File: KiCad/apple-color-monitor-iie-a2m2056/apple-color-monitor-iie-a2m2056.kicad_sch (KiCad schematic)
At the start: 395 parts, among them CN14 Conn_01x04_Pin, CN16 Conn_01x01_Pin, CN20 Conn_01x06_Pin, CN20_plug1 Conn_01x06, CN4 Conn_01x07_Pin, CN4_FRONT1 CN, CN5 Text/Gfx, CN5_FRONT1 Conn_01x02_Socket, CN6 GRN, CN8 Conn_01x02_Pin, CN9 Conn_01x01_Pin, IC102 CD4053B, J101 Jumper_2_Bridged, J102 Jumper_2_Bridged, J103 Jumper_2_Bridged, J104 Jumper_2_Bridged, J106 Jumper_2_Bridged, J107 Jumper_2_Bridged, J108 Jumper_2_Bridged, J109 Jumper_2_Bridged, J110 Jumper_2_Bridged, J111 Jumper_2_Bridged, J112 Jumper_2_Bridged, J113 Jumper_2_Bridged, J114 Jumper_2_Bridged, J126 Jumper_2_Bridged, J201 Jumper_2_Bridged, J202 Jumper_2_Bridged, J203 Jumper_2_Bridged, J204 Jumper_2_Bridged, J205 Jumper_2_Bridged, J302 Jumper_2_Bridged, J304 Jumper_2_Bridged, J306 Jumper_2_Bridged, J308 Jumper_2_Bridged, J401 Jumper_2_Bridged, J402 Jumper_2_Bridged, J603 Jumper_2_Bridged, J604 Jumper_2_Bridged, J801 Jumper_2_Bridged, J802 Jumper_2_Bridged, J803 Jumper_2_Bridged, J804 Jumper_2_Bridged, J805 Jumper_2_Bridged, J806 Jumper_2_Bridged, P701 VIDEO IN, Q101 C945, Q102 A733, Q103 A733, Q104 C945, Q105 A733, Q111 A642, Q114 C945, Q201 C1507, Q202 D1398, Q501 A709, Q502 C1008, Q503 C3042, Q504 A709, Q801 C945, Q802 C945, Q803 C945, Q804 A733, Q805 A733, Q806 A733, Q807 A733, Q808 A733, Q809 A733, SW1 SW_SPST, SW800 SVC_SW, T102 Transformer_1P_1S, T103 Transformer_1P_1S, T201 Transformer_1P_1S, T202 Transformer_1P_1S, T203 Transformer_SP_2S, T204 Fkyback, T205 Transformer_1P_1S, T501 Transformer_4_5_Unknwon, X102 DL401F5, X103 Crystal

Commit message: checkpoint
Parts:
- Q202: symbol Transistor_BJT:Q_NPN_BCE -> -my-symbols:_Power_Transistor_NPN_D1398
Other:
- moved on the sheet: C104, C105, C106, C112, C222, C223, C224, C225, C226, C229, C230, C502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

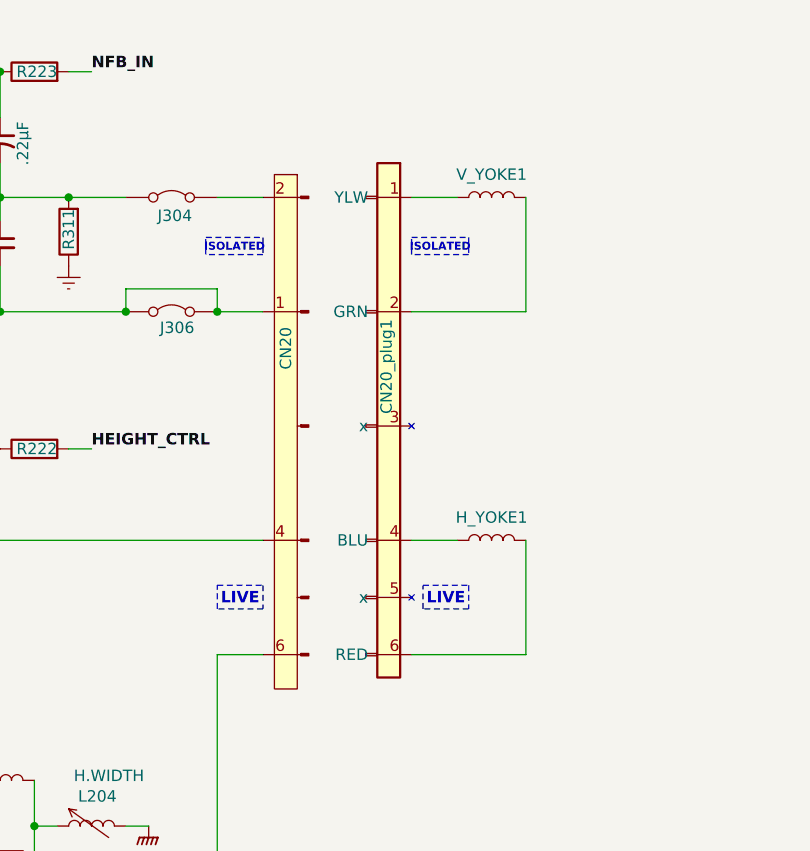
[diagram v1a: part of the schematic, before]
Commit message: checkpoint
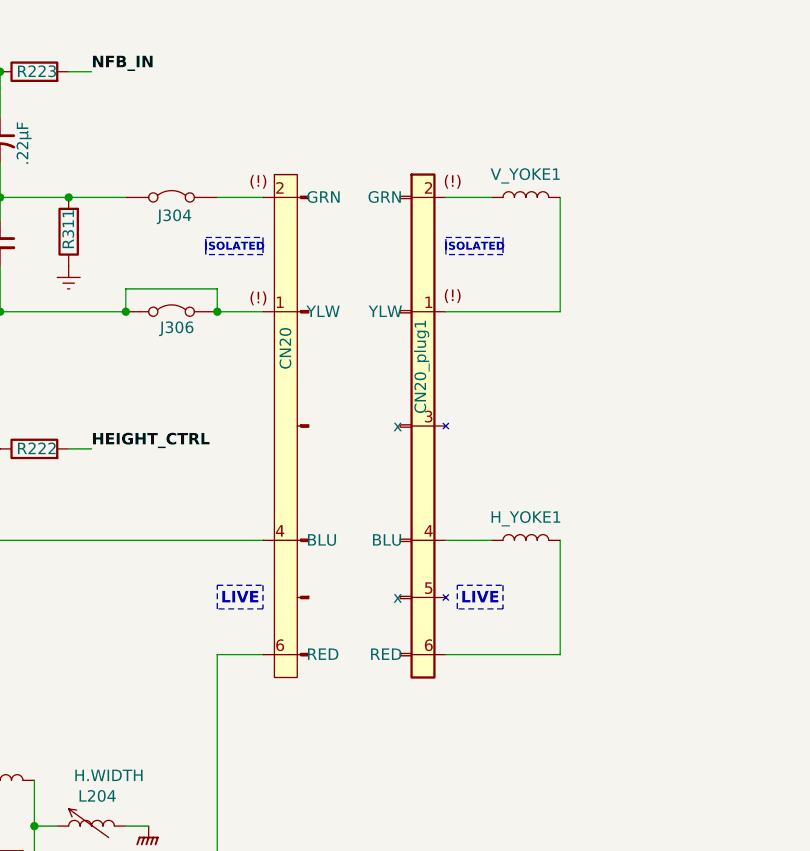
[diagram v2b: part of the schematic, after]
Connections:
- net at V_YOKE1.1: now also CN20_plug1.2 (GRN); no longer CN20_plug1.1 (YLW)
- net at V_YOKE1.2: now also CN20_plug1.1 (YLW); no longer CN20_plug1.2 (GRN)
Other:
- moved on the sheet: H_YOKE1, V_YOKE1
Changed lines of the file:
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@@
 	(text_box "ISOLATED"
 		(exclude_from_sim no)
-		(at 801.37 504.825 0)
+		(at 805.18 504.825 0)
 		(size 6.35 1.905)
 		(margins 0.127 0.127 0.127 0.127)
@@
 	(text_box "LIVE"
 		(exclude_from_sim no)
-		(at 802.64 543.4686 0)
+		(at 806.45 543.4686 0)
 		(size 5.08 2.6314)
 		(margins 0.127 0.127 0.127 0.127)
@@
 	(wire
 		(pts
-			(xy 814.07 538.48) (xy 814.07 551.18)
+			(xy 817.88 538.48) (xy 817.88 551.18)
 		)
 		(stroke
@@
 	(wire
 		(pts
-			(xy 806.45 500.38) (xy 801.37 500.38)
+			(xy 810.26 500.38) (xy 805.18 500.38)
 		)
 		(stroke
@@
 	(wire
 		(pts
-			(xy 814.07 500.38) (xy 814.07 513.08)
+			(xy 817.88 500.38) (xy 817.88 513.08)
 		)
 		(stroke
@@
 	(wire
 		(pts
-			(xy 814.07 513.08) (xy 801.37 513.08)
+			(xy 817.88 513.08) (xy 805.18 513.08)
 		)
 		(stroke
@@
 	(wire
 		(pts
-			(xy 814.07 551.18) (xy 801.37 551.18)
+			(xy 817.88 551.18) (xy 805.18 551.18)
 		)
 		(stroke
@@
 	(wire
 		(pts
-			(xy 801.37 538.48) (xy 806.45 538.48)
+			(xy 805.18 538.48) (xy 810.26 538.48)
 		)
 		(stroke
@@
 	(symbol
 		(lib_id "Device:L")
-		(at 810.26 538.48 90)
+		(at 814.07 538.48 90)
 		(unit 1)
 		(body_style 1)
@@
 		(fields_autoplaced yes)
 		(property "Reference" "H_YOKE1"
-			(at 810.26 535.94 90)
+			(at 814.07 535.94 90)
 			(show_name no)
 			(do_not_autoplace no)
@@
 		)
 		(property "Value" "L"
-			(at 811.5299 537.21 0)
+			(at 815.3399 537.21 0)
 			(hide yes)
 			(show_name no)
@@
 		)
 		(property "Footprint" ""
-			(at 810.26 538.48 0)
+			(at 814.07 538.48 0)
 			(hide yes)
 			(show_name no)
@@
 		)
 		(property "Datasheet" ""
-			(at 810.26 538.48 0)
+			(at 814.07 538.48 0)
 			(hide yes)
 			(show_name no)
@@
 		)
 		(property "Description" "Inductor"
-			(at 810.26 538.48 0)
+			(at 814.07 538.48 0)
 			(hide yes)
 			(show_name no)
@@
 	(symbol
 		(lib_id "Connector:Conn_01x06_Pin")
-		(at 789.94 525.78 0)
-		(mirror y)
+		(at 787.4 525.78 0)
 		(unit 1)
 		(body_style 1)
@@
 		)
 		(property "Value" "Conn_01x06_Pin"
-			(at 789.305 517.398 0)
+			(at 788.035 517.398 0)
 			(hide yes)
 			(show_name no)
@@
 		)
 		(property "Footprint" "_my-footprints:_CN20_pins"
-			(at 789.94 525.78 0)
+			(at 787.4 525.78 0)
 			(hide yes)
 			(show_name no)
@@
 		)
 		(property "Description" "Generic connector, single row, 01x06, script generated"
-			(at 789.94 525.78 0)
+			(at 787.4 525.78 0)
 			(hide yes)
 			(show_name no)
@@
 	(symbol
 		(lib_id "Device:L")
-		(at 810.26 500.38 90)
+		(at 814.07 500.38 90)
 		(unit 1)
 		(body_style 1)
@@
 		(fields_autoplaced yes)
 		(property "Reference" "V_YOKE1"
-			(at 810.26 497.84 90)
+			(at 814.07 497.84 90)
 			(show_name no)
 			(do_not_autoplace no)
@@
 		)
 		(property "Value" "L"
-			(at 811.5299 499.11 0)
+			(at 815.3399 499.11 0)
 			(hide yes)
 			(show_name no)
@@
 		)
 		(property "Footprint" ""
-			(at 810.26 500.38 0)
+			(at 814.07 500.38 0)
 			(hide yes)
 			(show_name no)
@@
 		)
 		(property "Datasheet" ""
-			(at 810.26 500.38 0)
+			(at 814.07 500.38 0)
 			(hide yes)
 			(show_name no)
@@
 		)
 		(property "Description" "Inductor"
-			(at 810.26 500.38 0)
+			(at 814.07 500.38 0)
 			(hide yes)
 			(show_name no)
@@
 	(symbol
 		(lib_id "Connector_Generic:Conn_01x06")
-		(at 796.29 525.78 0)
-		(mirror y)
+		(at 802.64 525.78 0)
 		(unit 1)
 		(body_style 1)
@@
 		(dnp no)
 		(property "Reference" "CN20_plug1"
-			(at 798.576 519.176 90)
+			(at 802.386 519.176 90)
 			(show_name no)
 			(do_not_autoplace no)
@@
 		)
 		(property "Value" "Conn_01x06"
-			(at 796.29 516.89 0)
+			(at 802.64 516.89 0)
 			(hide yes)
 			(show_name no)
@@
 		)
 		(property "Footprint" ""
-			(at 796.29 525.78 0)
+			(at 800.1 525.78 0)
 			(hide yes)
 			(show_name no)
@@
 		)
 		(property "Datasheet" ""
-			(at 796.29 525.78 0)
+			(at 800.1 525.78 0)
 			(hide yes)
 			(show_name no)
@@
 		)
 		(property "Description" "Generic connector, single row, 01x06, script generated (kicad-library-utils/schlib/autogen/connector/)"
-			(at 796.29 525.78 0)
+			(at 802.64 525.78 0)
 			(hide yes)
 			(show_name no)
